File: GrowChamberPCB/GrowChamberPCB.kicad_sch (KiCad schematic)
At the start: 3 parts, among them P1 12V_In, P3 Screw Terminal

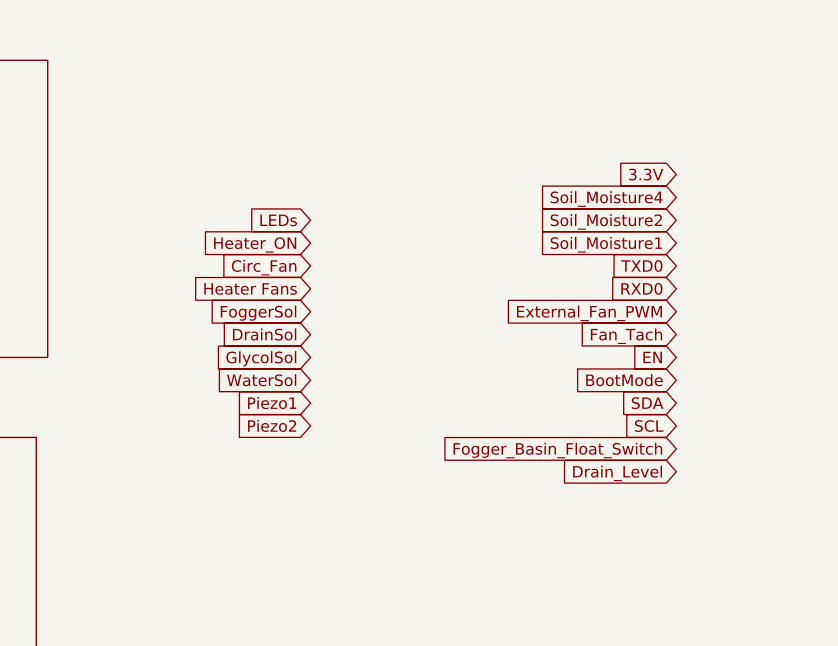
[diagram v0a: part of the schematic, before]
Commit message: almost done routing
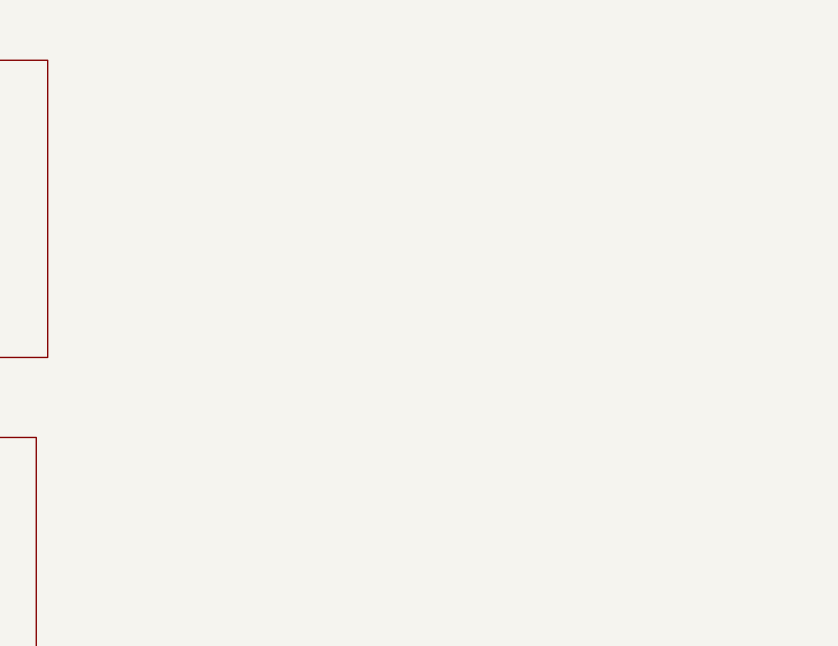
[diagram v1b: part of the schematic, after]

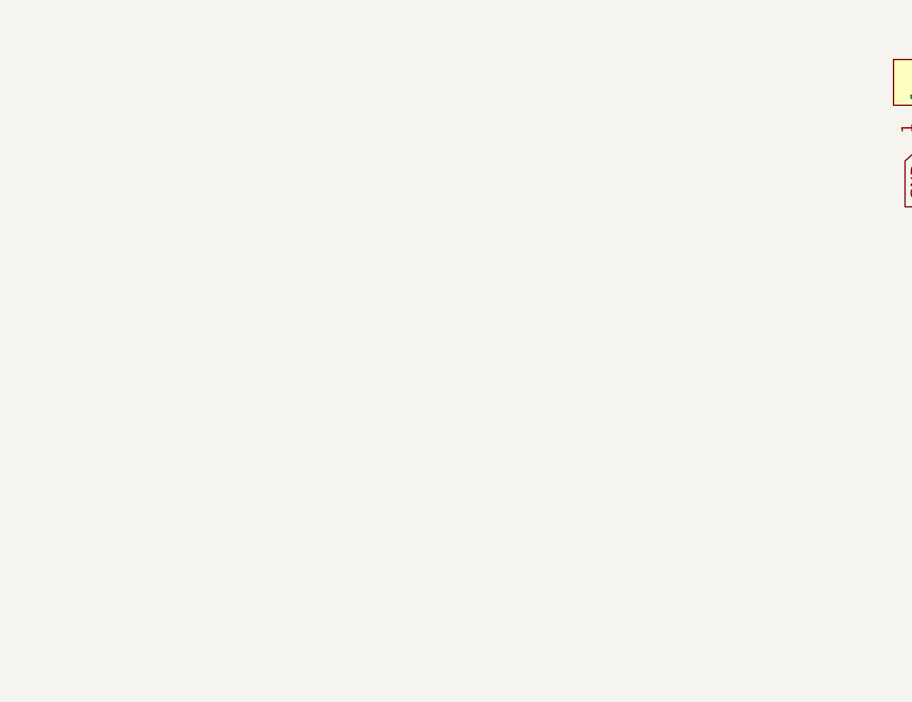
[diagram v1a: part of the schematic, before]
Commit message: redesign 3
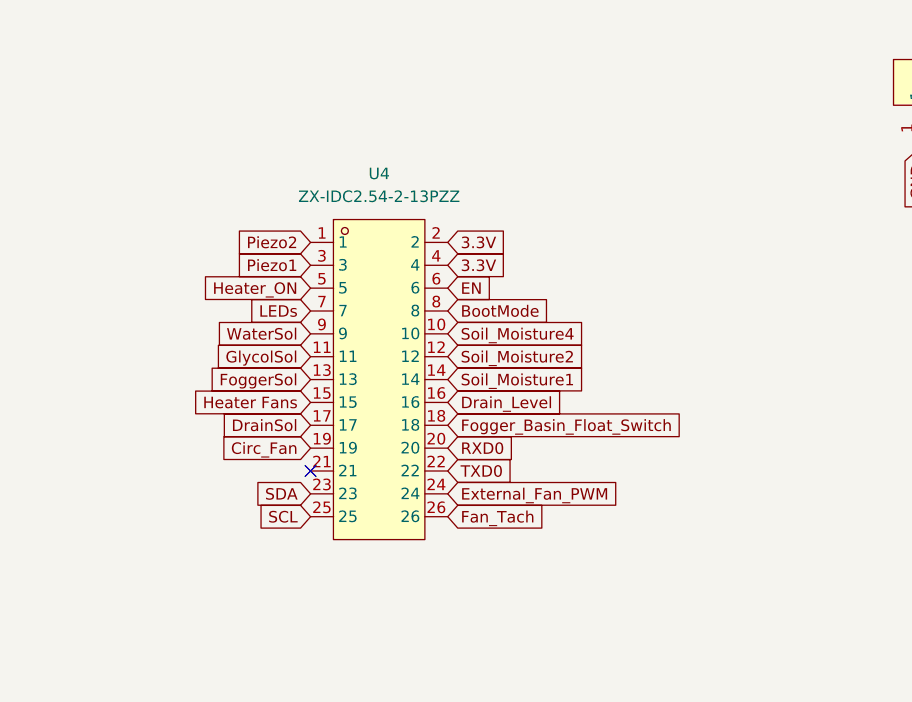
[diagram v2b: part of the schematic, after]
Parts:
- added U4: ZX-IDC2.54-2-13PZZ, easyeda2kicad:IDC-TH_26P-P2.54_ZX-IDC2.54-2-13PZZ, symbol easyeda2kicad:ZX-IDC2.54-2-13PZZ
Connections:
- net LEDs: now also U4.7
- new net 3.3V: U4.2, U4.4
- new net BootMode: U4.8
- new net Circ_Fan: U4.19
- new net DrainSol: U4.17
- new net Drain_Level: U4.16
- new net EN: U4.6
- new net External_Fan_PWM: U4.24
- new net Fan_Tach: U4.26
- new net FoggerSol: U4.13
- new net Fogger_Basin_Float_Switch: U4.18
- new net GlycolSol: U4.11
- new net Heater Fans: U4.15
- new net Heater_ON: U4.5
- new net Piezo1: U4.3
- new net Piezo2: U4.1
- new net RXD0: U4.20
- new net SCL: U4.25
- new net SDA: U4.23
- new net Soil_Moisture1: U4.14
- new net Soil_Moisture2: U4.12
- new net Soil_Moisture4: U4.10
- new net TXD0: U4.22
- new net WaterSol: U4.9
- no-connect marks 0 -> 1

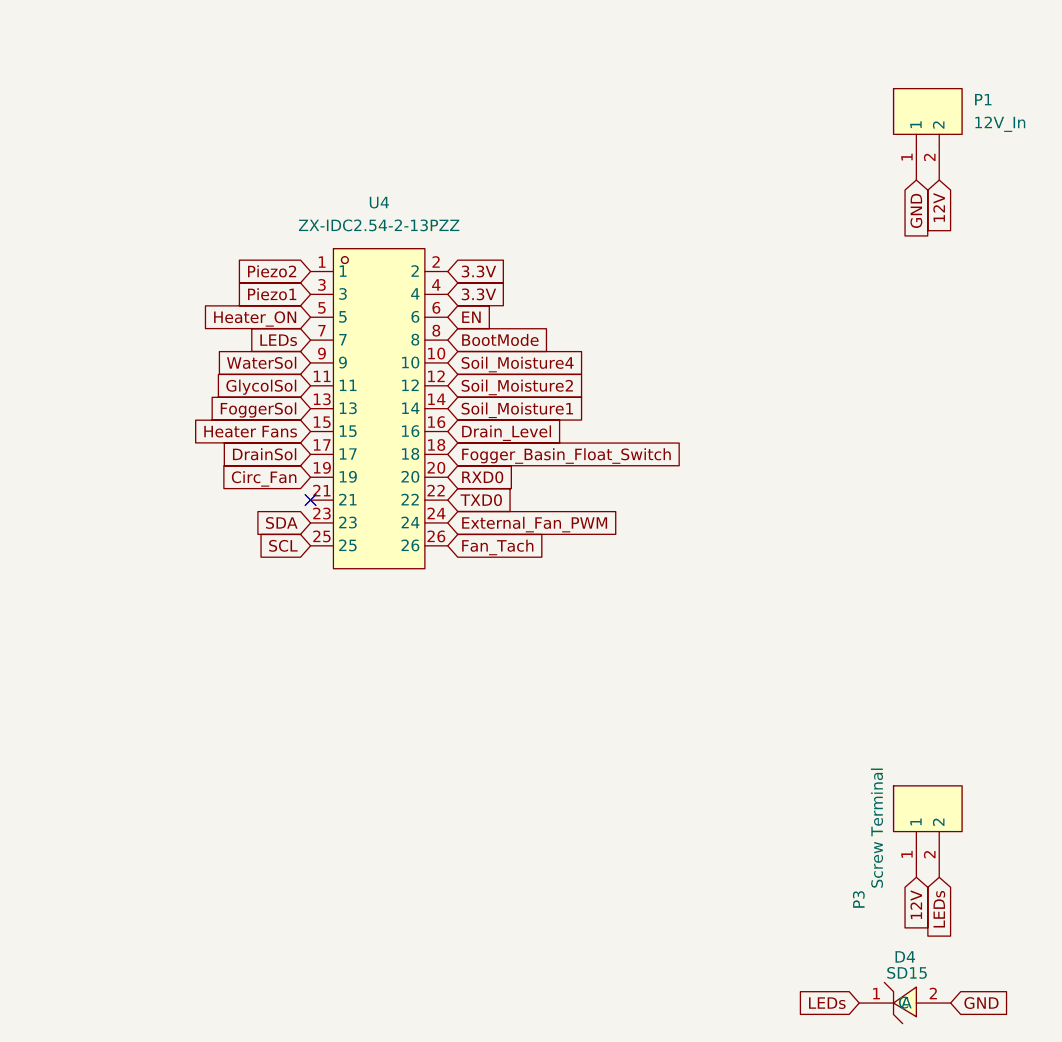
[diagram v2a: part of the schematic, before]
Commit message: finished routing
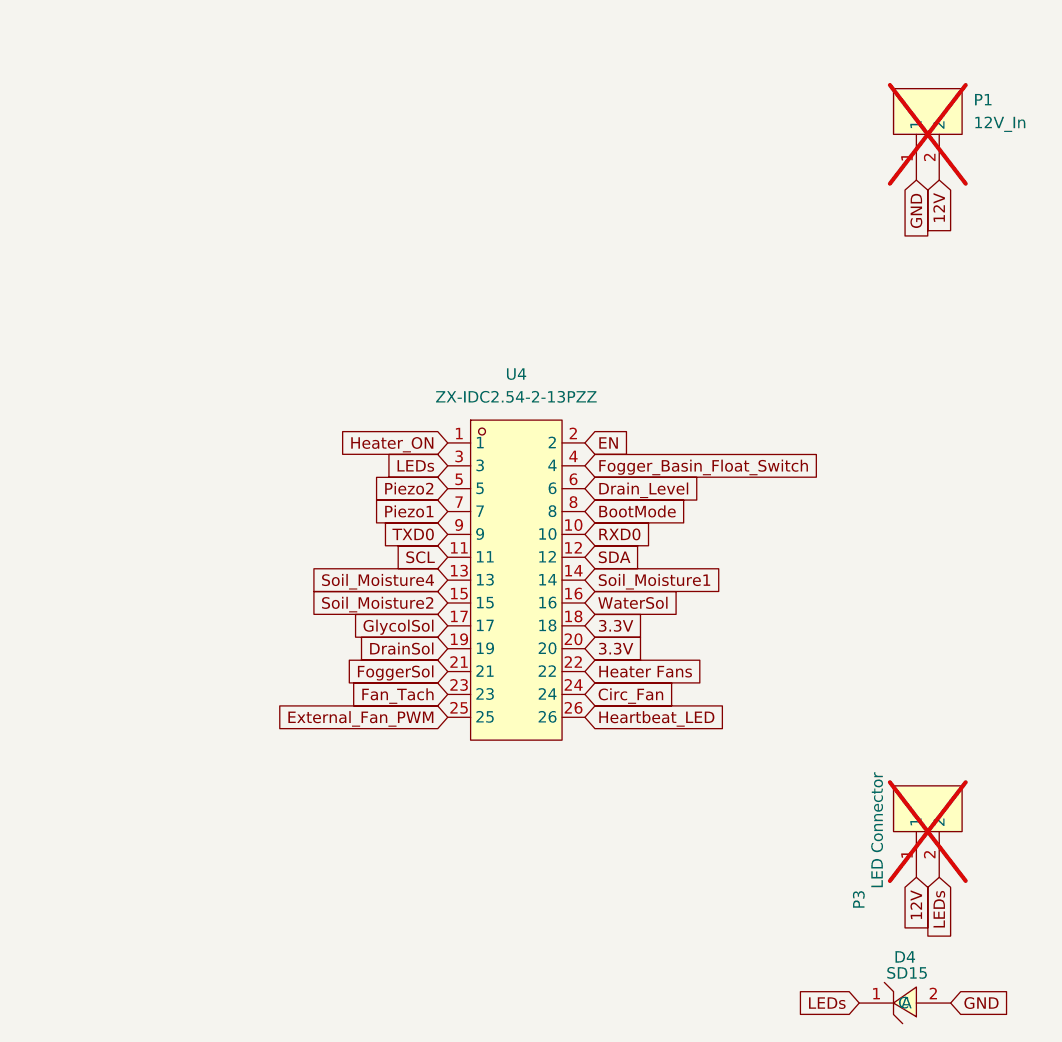
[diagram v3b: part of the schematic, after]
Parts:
- P1: now not fitted
- P3: value Screw Terminal -> LED Connector; now not fitted
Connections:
- net 3.3V: now also U4.18, U4.20; no longer U4.2, U4.4
- net Circ_Fan: now also U4.24; no longer U4.19
- net DrainSol: now also U4.19; no longer U4.17
- net Drain_Level: now also U4.6; no longer U4.16
- net EN: now also U4.2; no longer U4.6
- net External_Fan_PWM: now also U4.25; no longer U4.24
- net Fan_Tach: now also U4.23; no longer U4.26
- net FoggerSol: now also U4.21; no longer U4.13
- net Fogger_Basin_Float_Switch: now also U4.4; no longer U4.18
- net GlycolSol: now also U4.17; no longer U4.11
- net Heater Fans: now also U4.22; no longer U4.15
- net Heater_ON: now also U4.1; no longer U4.5
- net LEDs: now also U4.3; no longer U4.7
- net Piezo1: now also U4.7; no longer U4.3
- net Piezo2: now also U4.5; no longer U4.1
- net RXD0: now also U4.10; no longer U4.20
- net SCL: now also U4.11; no longer U4.25
- net SDA: now also U4.12; no longer U4.23
- net Soil_Moisture2: now also U4.15; no longer U4.12
- net Soil_Moisture4: now also U4.13; no longer U4.10
- net TXD0: now also U4.9; no longer U4.22
- net WaterSol: now also U4.16; no longer U4.9
- new net Heartbeat_LED: U4.26
- no-connect marks 1 -> 0
